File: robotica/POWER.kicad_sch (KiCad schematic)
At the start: 5 parts, among them J14 12V, J6 12V, U2 LM7805_TO220

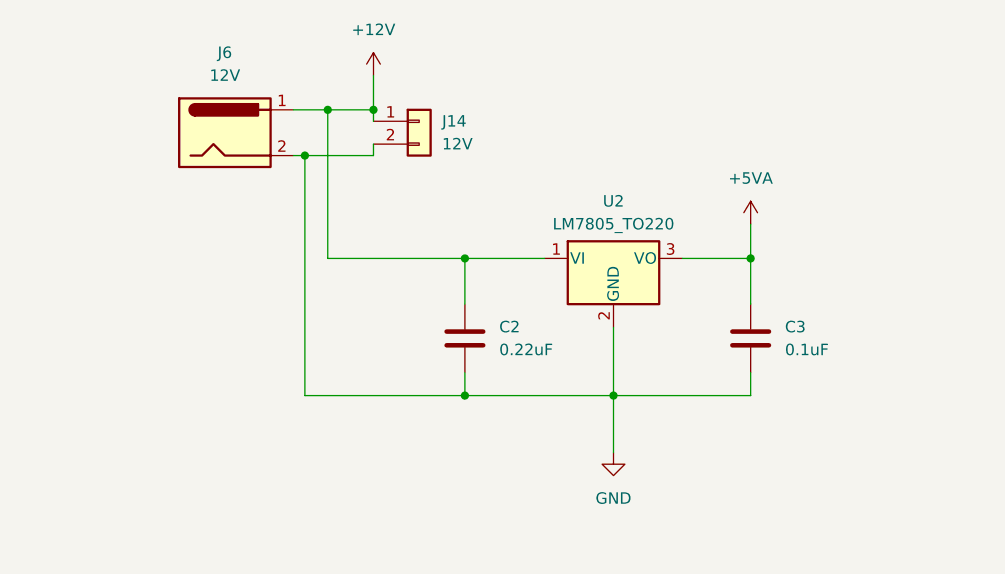
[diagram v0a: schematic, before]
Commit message: PCB YA REALIZADO
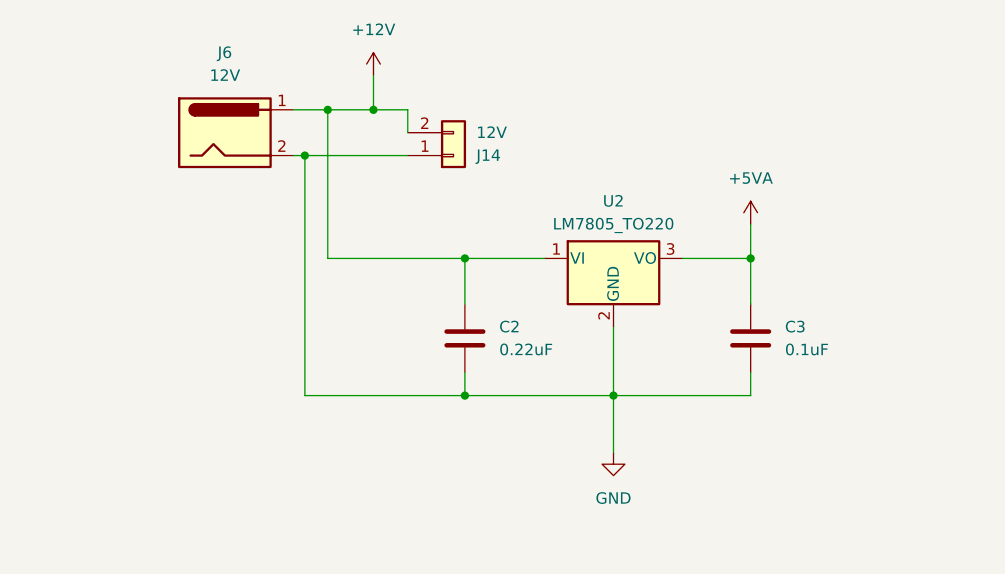
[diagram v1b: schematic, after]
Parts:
- C2: footprint (none) -> Capacitor_THT:C_Disc_D5.1mm_W3.2mm_P5.00mm
- C3: footprint (none) -> Capacitor_THT:C_Disc_D5.0mm_W2.5mm_P5.00mm
- J14: footprint (none) -> TerminalBlock:TerminalBlock_bornier-2_P5.08mm
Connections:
- net +12V: now also J14.2 (Pin_2); no longer J14.1 (Pin_1)
- net GND: now also J14.1 (Pin_1); no longer J14.2 (Pin_2)
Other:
- moved on the sheet: J14
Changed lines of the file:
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@@
   (junction (at 158.75 114.3) (diameter 0) (color 0 0 0 0)
   )
+  (junction (at 142.24 99.06) (diameter 0) (color 0 0 0 0)
+  )
   (junction (at 132.08 82.55) (diameter 0) (color 0 0 0 0)
   )
-  (junction (at 142.24 99.06) (diameter 0) (color 0 0 0 0)
-  )
   (junction (at 173.99 99.06) (diameter 0) (color 0 0 0 0)
   )
@@
     (stroke (width 0) (type default))
   )
+  (wire (pts (xy 124.46 87.63) (xy 135.89 87.63))
+    (stroke (width 0) (type default))
+  )
   (wire (pts (xy 173.99 114.3) (xy 158.75 114.3))
     (stroke (width 0) (type default))
   )
-  (wire (pts (xy 124.46 87.63) (xy 132.08 87.63))
-    (stroke (width 0) (type default))
-  )
   (wire (pts (xy 173.99 104.14) (xy 173.99 99.06))
     (stroke (width 0) (type default))
@@
     (stroke (width 0) (type default))
   )
-  (wire (pts (xy 132.08 87.63) (xy 132.08 86.36))
+  (wire (pts (xy 135.89 82.55) (xy 132.08 82.55))
     (stroke (width 0) (type default))
   )
@@
     (stroke (width 0) (type default))
   )
-  (wire (pts (xy 132.08 82.55) (xy 132.08 83.82))
-    (stroke (width 0) (type default))
-  )
   (wire (pts (xy 173.99 99.06) (xy 166.37 99.06))
     (stroke (width 0) (type default))
@@
     (stroke (width 0) (type default))
   )
+  (wire (pts (xy 135.89 85.09) (xy 135.89 82.55))
+    (stroke (width 0) (type default))
+  )
   (symbol (lib_id "power:GND") (at 158.75 120.65 0) (unit 1)
     (in_bom yes) (on_board yes) (dnp no) (fields_autoplaced)
@@
       (effects (font (size 1.27 1.27)) (justify left))
     )
-    (property "Footprint" "" (at 174.9552 111.76 0)
+    (property "Footprint" "Capacitor_THT:C_Disc_D5.0mm_W2.5mm_P5.00mm" (at 174.9552 111.76 0)
       (effects (font (size 1.27 1.27)) hide)
     )
@@
       (effects (font (size 1.27 1.27)) (justify left))
     )
-    (property "Footprint" "" (at 143.2052 111.76 0)
+    (property "Footprint" "Capacitor_THT:C_Disc_D5.1mm_W3.2mm_P5.00mm" (at 143.2052 111.76 0)
       (effects (font (size 1.27 1.27)) hide)
     )
@@
     )
   )
-  (symbol (lib_id "Connector_Generic:Conn_01x02") (at 137.16 83.82 0) (unit 1)
-    (in_bom yes) (on_board yes) (dnp no) (fields_autoplaced)
-    (property "Reference" "J14" (at 139.7 83.82 0)
-      (effects (font (size 1.27 1.27)) (justify left))
-    )
-    (property "Value" "12V" (at 139.7 86.36 0)
-      (effects (font (size 1.27 1.27)) (justify left))
-    )
-    (property "Footprint" "" (at 137.16 83.82 0)
-      (effects (font (size 1.27 1.27)) hide)
-    )
-    (property "Datasheet" "~" (at 137.16 83.82 0)
-      (effects (font (size 1.27 1.27)) hide)
-    )
+  (symbol (lib_id "Connector_Generic:Conn_01x02") (at 140.97 87.63 0) (mirror x) (unit 1)
+    (in_bom yes) (on_board yes) (dnp no)
+    (property "Reference" "J14" (at 143.51 87.63 0)
+      (effects (font (size 1.27 1.27)) (justify left))
+    )
+    (property "Value" "12V" (at 143.51 85.09 0)
+      (effects (font (size 1.27 1.27)) (justify left))
+    )
+    (property "Footprint" "TerminalBlock:TerminalBlock_bornier-2_P5.08mm" (at 140.97 87.63 0)
+      (effects (font (size 1.27 1.27)) hide)
+    )
+    (property "Datasheet" "~" (at 140.97 87.63 0)
+      (effects (font (size 1.27 1.27)) hide)
+    )

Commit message: termincacion del pcb de robotica
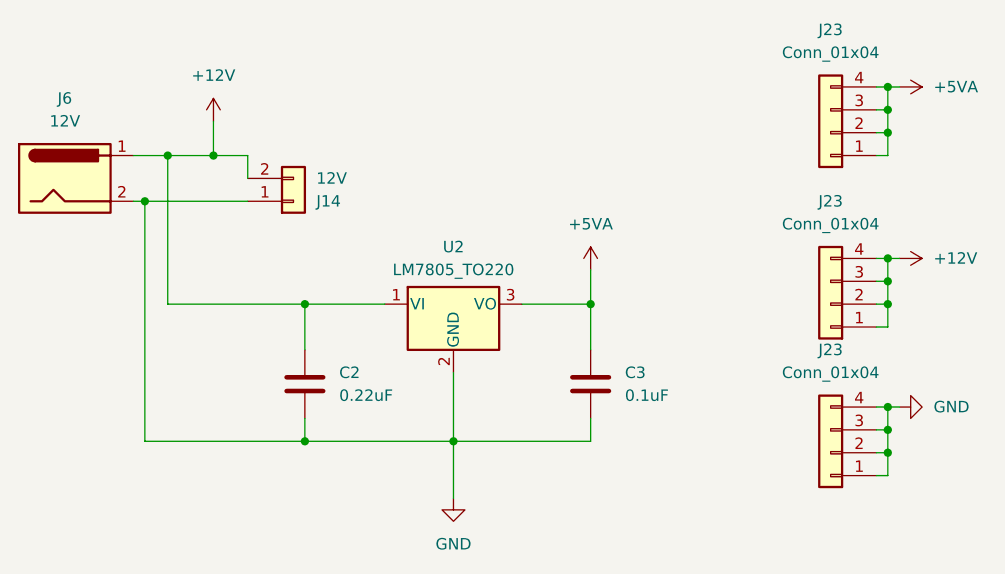
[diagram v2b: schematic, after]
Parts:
- added J23 (x3): Conn_01x04, Connector_PinSocket_2.54mm:PinSocket_1x04_P2.54mm_Vertical, symbol Connector_Generic:Conn_01x04
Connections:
- net +12V: now also J23.1 (Pin_1), J23.2 (Pin_2), J23.3 (Pin_3), J23.4 (Pin_4)
- net +5VA: now also J23.1 (Pin_1), J23.2 (Pin_2), J23.3 (Pin_3), J23.4 (Pin_4)
- net GND: now also J23.1 (Pin_1), J23.2 (Pin_2), J23.3 (Pin_3), J23.4 (Pin_4)
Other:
- moved on the sheet: C2, C3, J14, J6, U2
